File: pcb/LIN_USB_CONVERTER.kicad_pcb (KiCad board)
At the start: 2 copper layers, 17.8 x 34 mm, 32 parts, among them J1 Conn_01x03, J2 Conn_01x03, J3 GS2, J4 USB_A, J5 Conn_01x02, P2 CONN_01X05, U1 TJA1028, U2 MAX12931, U3 MCP1700T-3302E/TT, U4 STM32F042G4U6

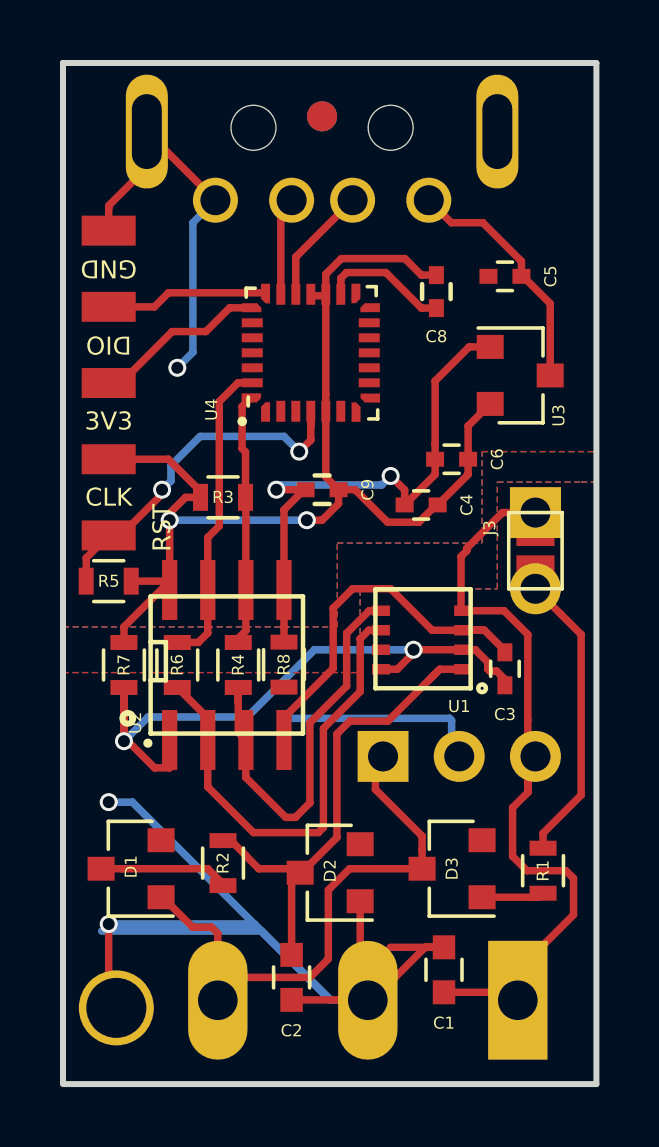
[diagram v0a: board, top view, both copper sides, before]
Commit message: Kicad update
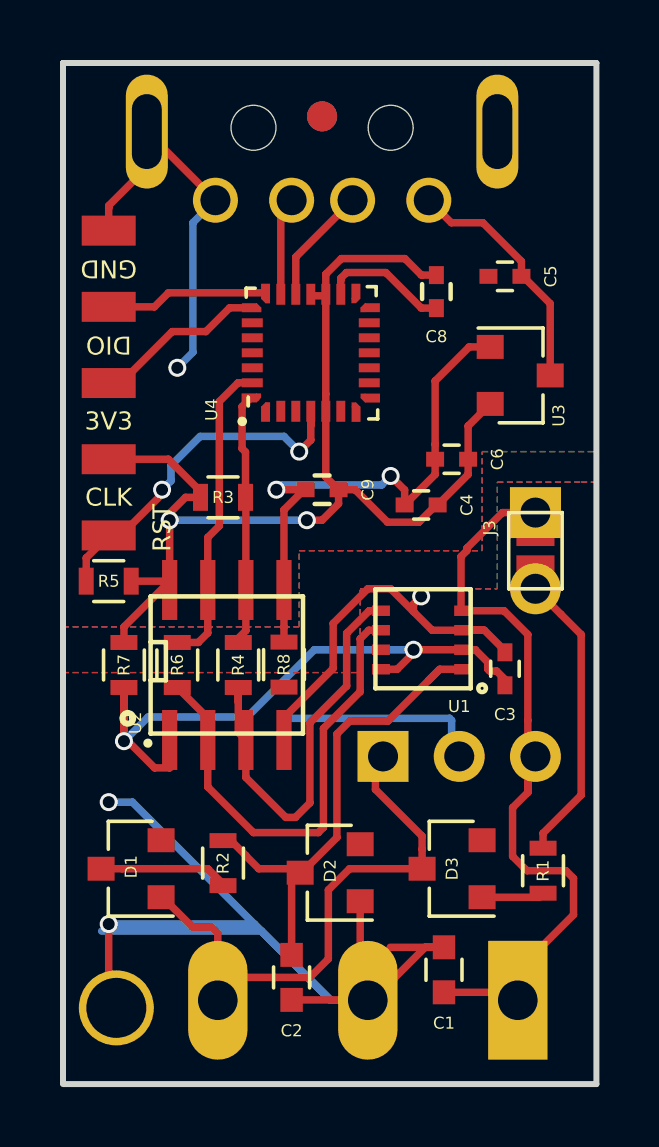
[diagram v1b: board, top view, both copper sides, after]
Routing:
- net -BATT: track 62.3 -> 62.7 mm, vias 2 -> 3
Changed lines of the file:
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@@
-(kicad_pcb (version 4) (host pcbnew 4.0.7)
+(kicad_pcb (version 20171130) (host pcbnew "(2018-02-16 revision c95340fba)-makepkg")
   (general
-    (links 84)
-    (no_connects 7)
-    (area 140.121999 78.203999 158.102001 112.440001)
     (thickness 1.6)
     (drawings 20)
-    (tracks 272)
+    (tracks 276)
     (zones 0)
     (modules 32)
@@
       (layerselection 0x3ffff_80000001)
       (usegerberextensions true)
+      (usegerberattributes false)
+      (usegerberadvancedattributes false)
+      (creategerberjobfile false)
       (excludeedgelayer true)
       (linewidth 0.100000)
@@
       (hpglpenspeed 20)
       (hpglpendiameter 15)
-      (hpglpenoverlay 2)
       (psnegative false)
       (psa4output false)
@@
     (tags "capacitor 0402")
     (attr smd)
-    (fp_text reference C8 (at 1.5 0 540) (layer F.SilkS)
+    (fp_text reference C8 (at 1.5 0 180) (layer F.SilkS)
       (effects (font (size 0.4 0.4) (thickness 0.09)))
     )
@@
     (tags "capacitor 0402")
     (attr smd)
-    (fp_text reference C3 (at 1.524 0 540) (layer F.SilkS)
+    (fp_text reference C3 (at 1.524 0 180) (layer F.SilkS)
       (effects (font (size 0.4 0.4) (thickness 0.09)))
     )
@@
     (tags "capacitor 0603")
     (attr smd)
-    (fp_text reference C2 (at 1.778 0 360) (layer F.SilkS)
+    (fp_text reference C2 (at 1.778 0) (layer F.SilkS)
       (effects (font (size 0.4 0.4) (thickness 0.09)))
     )
@@
     (tags "capacitor 0402")
     (attr smd)
-    (fp_text reference C6 (at -1.524 0 450) (layer F.SilkS)
+    (fp_text reference C6 (at -1.524 0 90) (layer F.SilkS)
       (effects (font (size 0.4 0.4) (thickness 0.09)))
     )
@@
     (descr "Through hole straight pin header, 1x03, 2.54mm pitch, single row")
     (tags "Through hole pin header THT 1x03 2.54mm single row")
-    (fp_text reference J1 (at 1.27 1.524 450) (layer B.SilkS)
+    (fp_text reference J1 (at 1.27 1.524 90) (layer B.SilkS)
       (effects (font (size 0.4 0.4) (thickness 0.09)) (justify mirror))
     )
@@
     (fp_line (start 1.8 -6.85) (end 1.8 1.8) (layer B.CrtYd) (width 0.05))
     (fp_line (start 1.8 1.8) (end -1.8 1.8) (layer B.CrtYd) (width 0.05))
-    (fp_text user %R (at 0 -2.54 540) (layer B.Fab)
+    (fp_text user %R (at 0 -2.54 180) (layer B.Fab)
       (effects (font (size 0.4 0.4) (thickness 0.09)) (justify mirror))
     )
@@
     (fp_line (start 1.8 -4.35) (end 1.8 1.8) (layer B.CrtYd) (width 0.05))
     (fp_line (start 1.8 1.8) (end -1.8 1.8) (layer B.CrtYd) (width 0.05))
-    (fp_text user %R (at 0 -1.27 450) (layer B.Fab)
+    (fp_text user %R (at 0 -1.27 90) (layer B.Fab)
       (effects (font (size 0.4 0.4) (thickness 0.09)) (justify mirror))
     )
@@
     (pad "" np_thru_hole circle (at 5.842 -2.413) (size 1.5 1.5) (drill 1.5) (layers *.Cu *.Mask))
     (model Connect.3dshapes/USB_A.wrl
-      (at (xyz 0.14 0 0))
+      (offset (xyz 3.555999946594238 0 0))
       (scale (xyz 1 1 1))
       (rotate (xyz 0 0 90))
@@
   (segment (start 156.462 86.324) (end 155.554 85.416) (width 0.25) (layer F.Cu) (net 8))
   (segment (start 155.554 85.416) (end 155.504 85.416) (width 0.25) (layer F.Cu) (net 8))
+  (segment (start 151.143002 95.83) (end 150.382 95.83) (width 0.25) (layer F.Cu) (net 9))
+  (segment (start 151.905002 96.592) (end 151.143002 95.83) (width 0.25) (layer F.Cu) (net 9))
+  (segment (start 150.382 95.83) (end 149.227978 96.984022) (width 0.25) (layer F.Cu) (net 9))
+  (segment (start 149.227978 96.984022) (end 149.227978 98.484022) (width 0.25) (layer F.Cu) (net 9))
+  (segment (start 149.227978 98.484022) (end 147.588 100.124) (width 0.25) (layer F.Cu) (net 9))
+  (segment (start 147.588 100.124) (end 147.588 100.87) (width 0.25) (layer F.Cu) (net 9))
+  (segment (start 151.905002 96.338998) (end 152.16 96.084) (width 0.25) (layer F.Cu) (net 9))
+  (via (at 152.16 96.084) (size 0.6) (drill 0.4) (layers F.Cu B.Cu) (net 9))
+  (segment (start 152.525002 97.212) (end 151.905002 96.592) (width 0.25) (layer F.Cu) (net 9))
+  (segment (start 151.905002 96.592) (end 151.905002 96.338998) (width 0.25) (layer F.Cu) (net 9))
   (segment (start 154.192 97.212) (end 153.56 97.212) (width 0.25) (layer F.Cu) (net 9))
-  (segment (start 147.588 100.124) (end 147.588 100.87) (width 0.25) (layer F.Cu) (net 9))
-  (segment (start 152.525002 97.212) (end 151.143002 95.83) (width 0.25) (layer F.Cu) (net 9))
-  (segment (start 149.227978 98.484022) (end 147.588 100.124) (width 0.25) (layer F.Cu) (net 9))
-  (segment (start 151.143002 95.83) (end 149.874 95.83) (width 0.25) (layer F.Cu) (net 9))
   (segment (start 154.192 97.212) (end 152.525002 97.212) (width 0.25) (layer F.Cu) (net 9))
-  (segment (start 149.874 95.83) (end 149.227978 96.476022) (width 0.25) (layer F.Cu) (net 9))
-  (segment (start 149.227978 96.476022) (end 149.227978 98.484022) (width 0.25) (layer F.Cu) (net 9))
   (segment (start 150.128 106.244) (end 150.128 109.292) (width 0.25) (layer F.Cu) (net 9))
   (segment (start 150.128 109.292) (end 150.382 109.546) (width 0.25) (layer F.Cu) (net 9))
@@
     (polygon
       (pts
-        (xy 140.222 97.1) (xy 149.366 97.1) (xy 149.366 94.306) (xy 154.192 94.306) (xy 154.192 91.258)
+        (xy 140.222 97.1) (xy 148.096 97.1) (xy 148.096 94.56) (xy 154.192 94.56) (xy 154.192 91.258)
         (xy 157.748 91.258) (xy 158.002 91.258) (xy 158.002 78.304) (xy 140.222 78.304)
       )
@@
     (polygon
       (pts
-        (xy 140.222 97.1) (xy 149.366 97.1) (xy 149.366 94.306) (xy 154.192 94.306) (xy 154.192 91.258)
+        (xy 140.222 97.1) (xy 148.096 97.1) (xy 148.096 94.56) (xy 154.192 94.56) (xy 154.192 91.258)
         (xy 157.748 91.258) (xy 158.002 91.258) (xy 158.002 78.304) (xy 140.222 78.304)
       )
